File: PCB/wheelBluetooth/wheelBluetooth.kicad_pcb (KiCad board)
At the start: 2 copper layers, 37 parts, among them J1 USB_C_Receptacle_USB2.0, J2 Conn_01x02_Male, J3 Conn_01x06_Male, J4 Conn_01x07_Male, J5 Conn_01x07_Male, Q1 A03401A, Q2 MBT3904DW1, SW1 SW_Push, SW2 SW_Push, SW3 SW_Push, SW4 SW_Push, SW5 SW_Push, SW6 SW_Push, SW7 SW_Push, U1 ESP32-WROOM-32, U2 MCP73831-5-OT, U3 XC6206P332MR

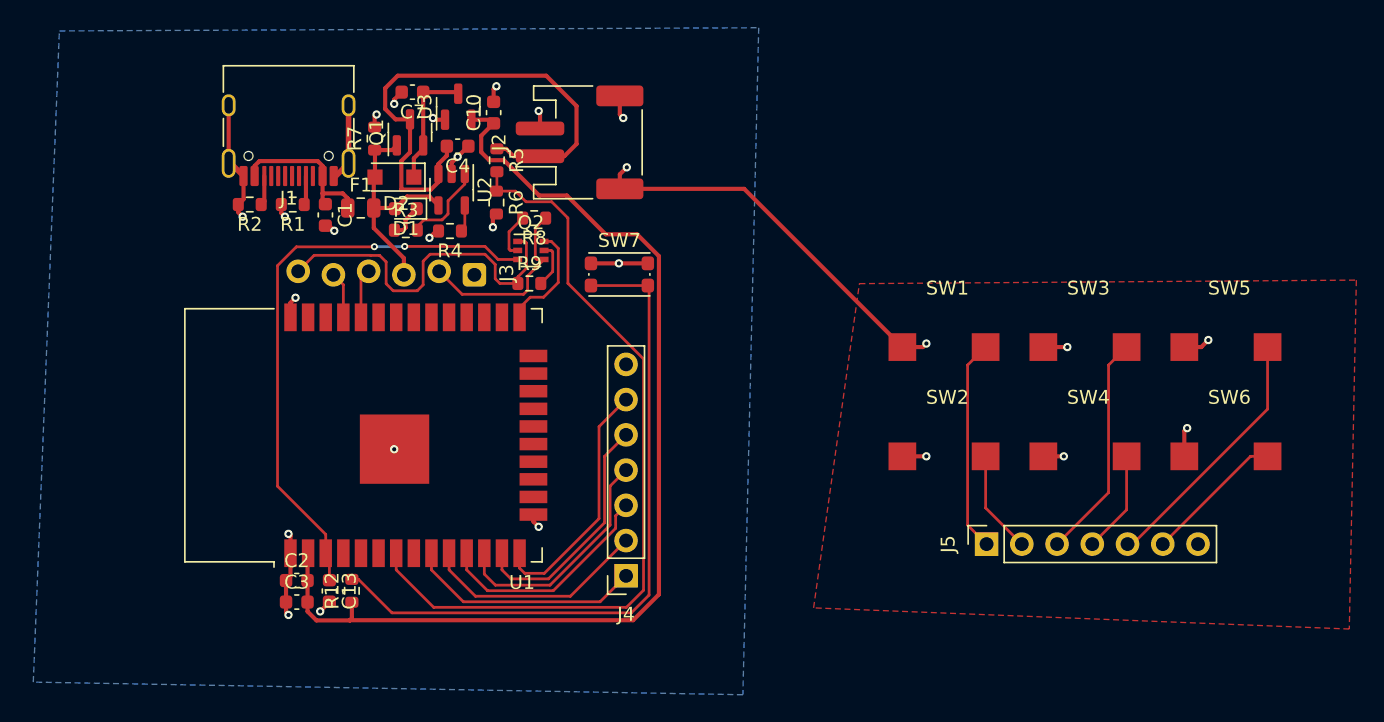
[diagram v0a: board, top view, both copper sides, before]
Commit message: Updated PCB
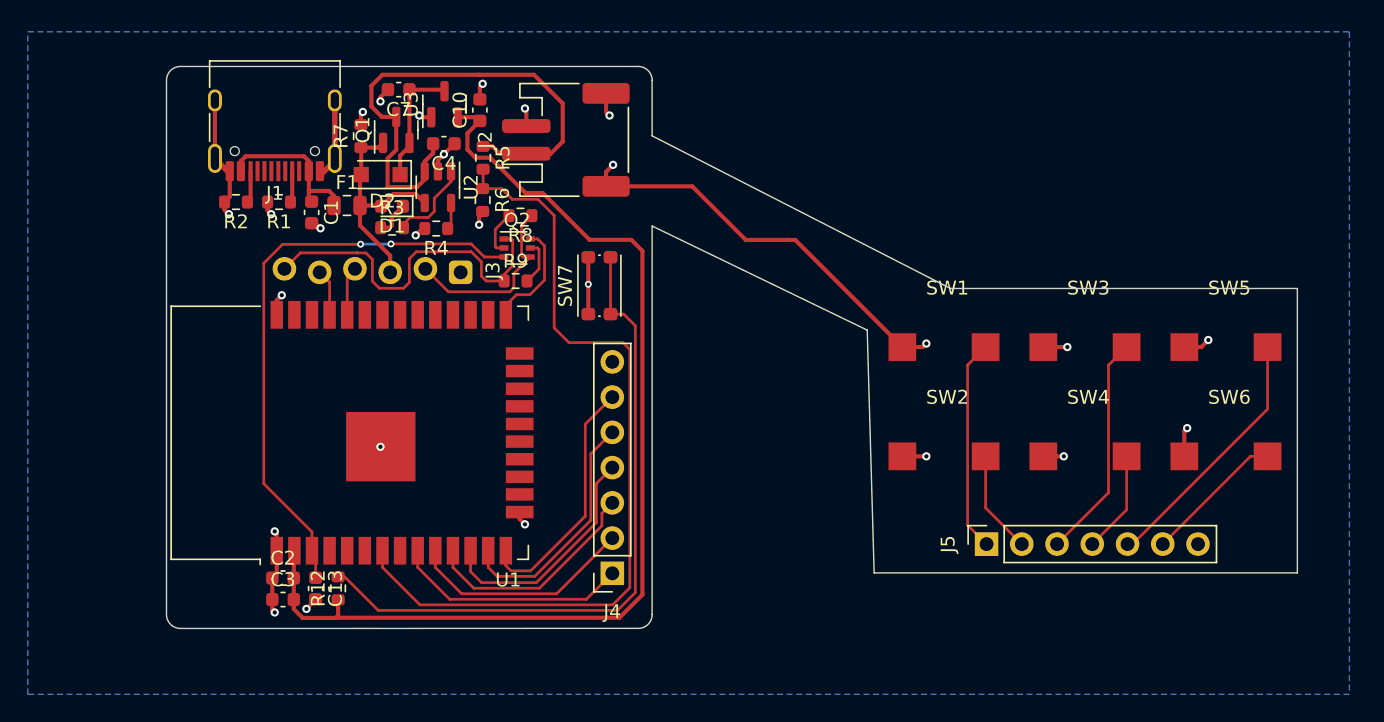
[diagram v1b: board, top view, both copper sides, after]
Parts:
- moved SW7 1.65 mm to (183.7, 73.3), turned to 90 degrees
- moved J1 1.05 mm to (160.3, 61.0)
- moved R12 1.01 mm to (164.9, 95.1)
- moved R4 1.01 mm to (171.9, 69.2)
- moved R6 1.01 mm to (175.3, 67.1)
- moved J2 1.01 mm to (181.3, 62.8)
- moved Q1 1.01 mm to (169.1, 62.1)
- moved C13 1.01 mm to (163.2, 95.1)
- moved D2 1.01 mm to (167.9, 65.3)
- moved U2 1.01 mm to (172.1, 66.2)
- moved C1 1.01 mm to (163.0, 68.0)
- moved C10 1.01 mm to (175.1, 60.6)
- moved C4 1.01 mm to (172.5, 63.1)
- moved C7 1.01 mm to (169.2, 59.2)
- moved D1 1.01 mm to (168.8, 67.6)
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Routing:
- net /VBAT: track 57.1 -> 59.4 mm
- net GND: track 79.3 -> 80.8 mm
- net Net-(R12-Pad2): track 49.4 -> 48.4 mm
- removed copper zone on F.Cu, net GND
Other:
- board outline added: 81.5 x 40.5 mm
